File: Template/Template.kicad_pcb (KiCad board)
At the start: 2 copper layers, 85 x 99.5 mm, 19 parts

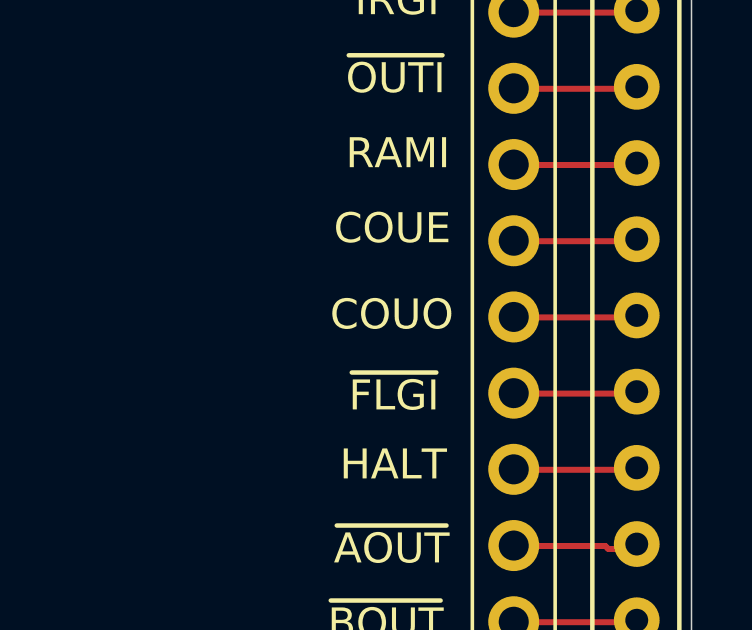
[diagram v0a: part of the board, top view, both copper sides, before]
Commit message: [Template] - updated for COUO being inverted signal  Please enter the commit message for your changes. Lines starting
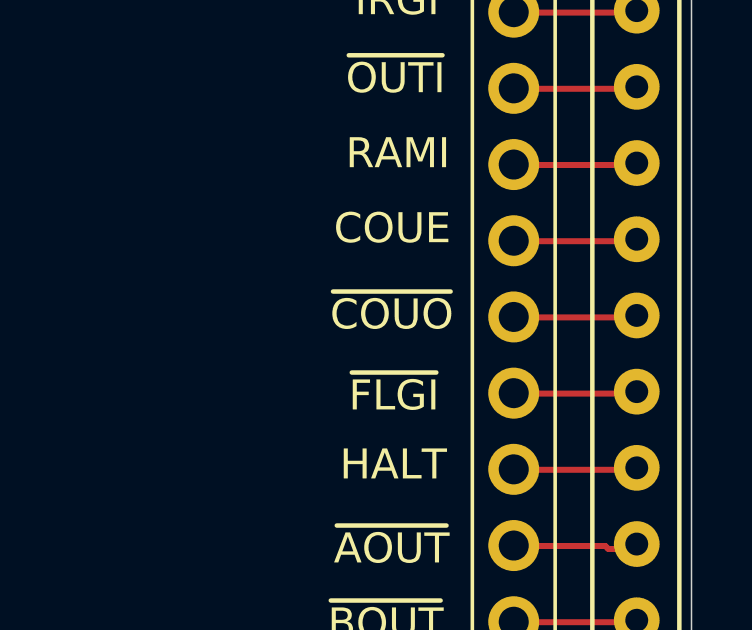
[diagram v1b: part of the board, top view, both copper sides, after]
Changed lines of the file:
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@@
 		(capping no)
 		(filling no)
-		(zone_defaults)
 		(pcbplotparams
 			(layerselection 0x00000000_00000000_55555555_5755f5ff)
@@
 			)
 		)
-		(fp_text user "COUO"
+		(fp_text user "~{COUO}"
 			(at 31.255 -12.785 0)
 			(unlocked yes)
@@
 	)
 	(segment
+		(start 25.62 107.46)
+		(end 28.845 107.46)
+		(width 0.2)
+		(layer "F.Cu")
+		(net "ZFLAG")
+	)
+	(segment
+		(start 28.845 107.46)
+		(end 29.325 107.94)
+		(width 0.2)
+		(layer "F.Cu")
+		(net "ZFLAG")
+	)
+	(segment
 		(start 28.845 110)
 		(end 29.325 110.48)
@@
 	)
 	(segment
+		(start 25.62 112.54)
+		(end 28.845 112.54)
+		(width 0.2)
+		(layer "F.Cu")
+		(net "ZFLAG2")
+	)
+	(segment
+		(start 28.845 112.54)
+		(end 29.325 113.02)
+		(width 0.2)
+		(layer "F.Cu")
+		(net "ZFLAG2")
+	)
+	(segment
+		(start 28.845 115.08)
+		(end 29.325 115.56)
+		(width 0.2)
+		(layer "F.Cu")
+		(net "CFLAG2")
+	)
+	(segment
+		(start 25.62 115.08)
+		(end 28.845 115.08)
+		(width 0.2)
+		(layer "F.Cu")
+		(net "CFLAG2")
+	)
+	(segment
 		(start 25.62 117.62)
 		(end 28.845 117.62)
@@
 		(net "Net-(D7-K)")
 	)
-	(segment
-		(start 25.62 107.46)
-		(end 28.845 107.46)
-		(width 0.2)
-		(layer "F.Cu")
-		(net "ZFLAG")
-	)
-	(segment
-		(start 28.845 107.46)
-		(end 29.325 107.94)
-		(width 0.2)
-		(layer "F.Cu")
-		(net "ZFLAG")
-	)
-	(segment
-		(start 28.845 115.08)
-		(end 29.325 115.56)
-		(width 0.2)
-		(layer "F.Cu")
-		(net "CFLAG2")
-	)
-	(segment
-		(start 25.62 115.08)
-		(end 28.845 115.08)
-		(width 0.2)
-		(layer "F.Cu")
-		(net "CFLAG2")
-	)
-	(segment
-		(start 25.62 112.54)
-		(end 28.845 112.54)
-		(width 0.2)
-		(layer "F.Cu")
-		(net "ZFLAG2")
-	)
-	(segment
-		(start 28.845 112.54)
-		(end 29.325 113.02)
-		(width 0.2)
-		(layer "F.Cu")
-		(net "ZFLAG2")
-	)
 	(embedded_fonts no)
